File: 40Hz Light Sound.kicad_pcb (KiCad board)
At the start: 2 copper layers, 49 x 30 mm, 8 parts, among them J1 11.1VDC, J2 DC2DC, J3 Audio_Amp, J4 LED_Conn, J5 AudioJack3_Ground, Q1 IRLZ44N, SW1 SW_SPDT, U1 ESP32-C3_SUPERMINI_TH

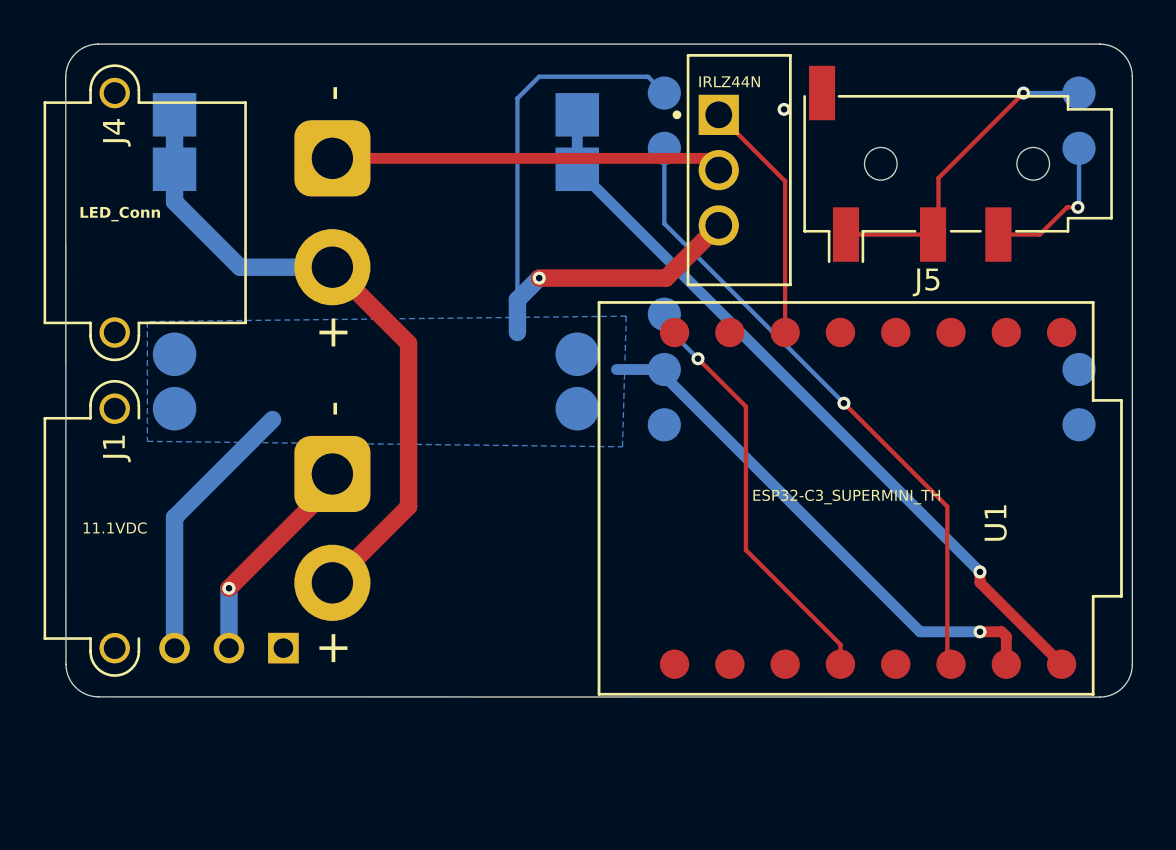
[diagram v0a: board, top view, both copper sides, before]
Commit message: Submit v0.1 to order
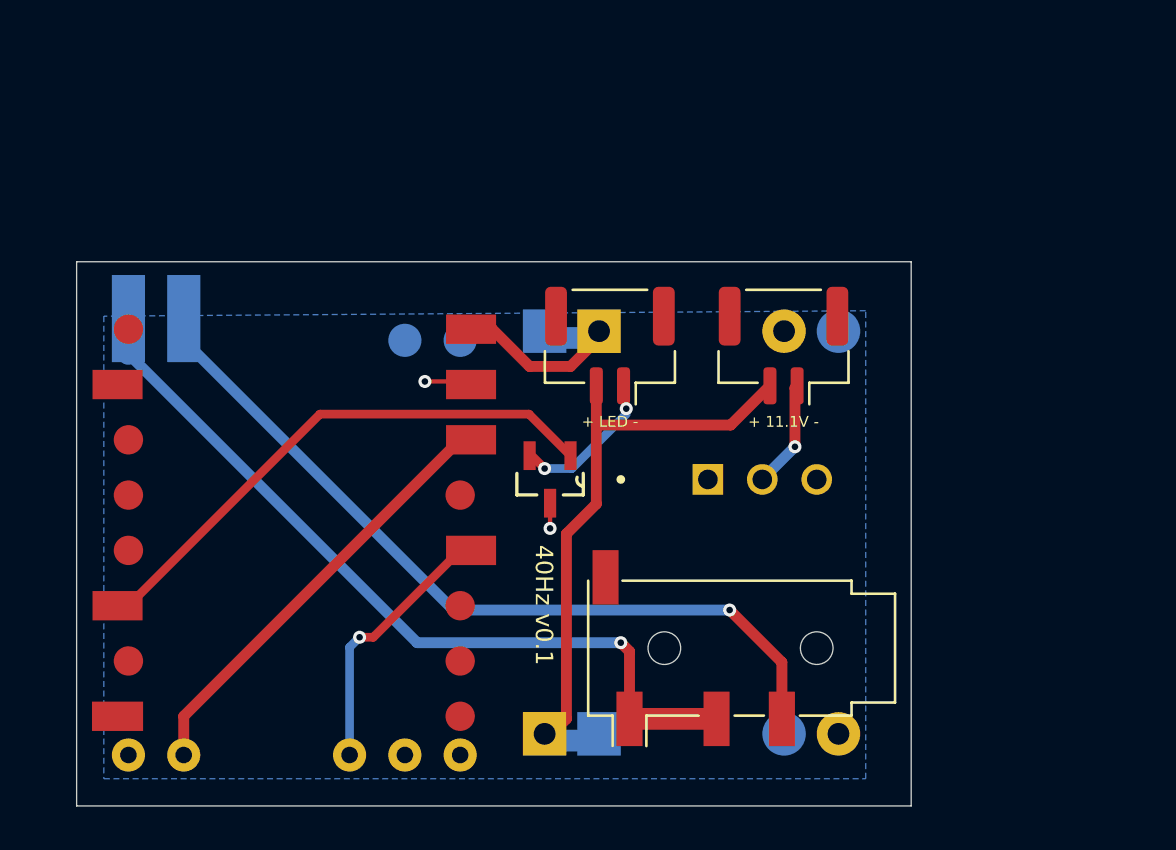
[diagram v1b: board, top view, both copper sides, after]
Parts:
- removed J1: 11.1VDC, Connector_AMASS:AMASS_XT30PW-M_1x02_P2.50mm_Horizontal
- removed J4: LED_Conn, Connector_AMASS:AMASS_XT30PW-M_1x02_P2.50mm_Horizontal
- added + 11.1V -: 11.1VDC, Connector_JST:JST_GH_SM02B-GHS-TB_1x02-1MP_P1.25mm_Horizontal, F.Cu at (182.0, 103.8)
- added + LED -: LED_Conn, Connector_JST:JST_GH_SM02B-GHS-TB_1x02-1MP_P1.25mm_Horizontal, F.Cu at (174.0, 103.8)
- Q1: value IRLZ44N -> IRLML6344; footprint IRLZ44N:TO254P1054X469X1930-3 -> IRLML6344TRPBF:SOT95P240X112-3N
- SW1: moved to F.Cu
- moved J2 36.2 mm to (169.2, 123.4), turned to 90 degrees
- moved J3 30.0 mm to (159.5, 112.5), turned to 180 degrees
- moved SW1 25.7 mm to (181.0, 110.0), turned to 0 degrees
- moved U1 25.4 mm to (159.5, 113.0), turned to 0 degrees
- moved J5 24.4 mm to (178.7, 117.8)
- moved Q1 16.7 mm to (171.2, 110.0)
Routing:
- net GND: track 65.5 -> 2.64 mm
- net Sound_N: track 6.65 -> 36.2 mm
- net 5VDC: track 34.5 -> 10.1 mm, vias 1 -> 0
- net Sound_P: track 14.7 -> 36.4 mm
- net LEDcontrol: track 11.3 -> 24.7 mm
- net LED_GND: track 19.7 -> 7.07 mm, vias 0 -> 2
- net 3.3V: track 29.2 -> 19.7 mm, vias 1 -> 0
- net SoundControl: track 19.6 -> 11.9 mm
- net 11.1V_GND: track 9.97 -> 4.96 mm
- net 11.1V: track 29.9 -> 29.1 mm
- net (no net): vias 1 -> 0
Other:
- board size 49 x 30 mm -> 38.3 x 25 mm
- board text added: "3.3V"
- board text added: "40Hz v0.1"
- board text added: "OUT"
- board text added: "Sound"
- board text added: "Sound+"
